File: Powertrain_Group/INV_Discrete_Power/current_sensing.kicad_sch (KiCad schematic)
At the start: 5 parts, among them U1 CKSR_75-NP

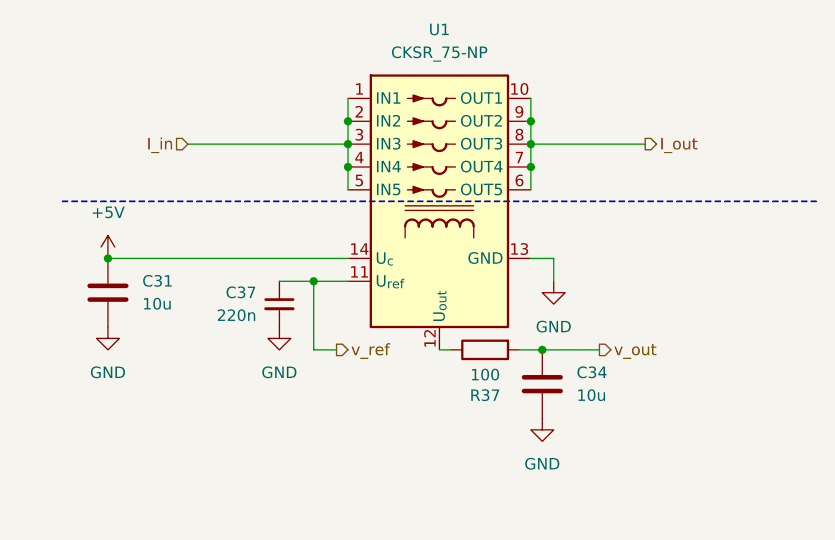
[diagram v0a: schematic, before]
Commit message: [INV_Discrete_Power] V1.1 by Jack Kuo
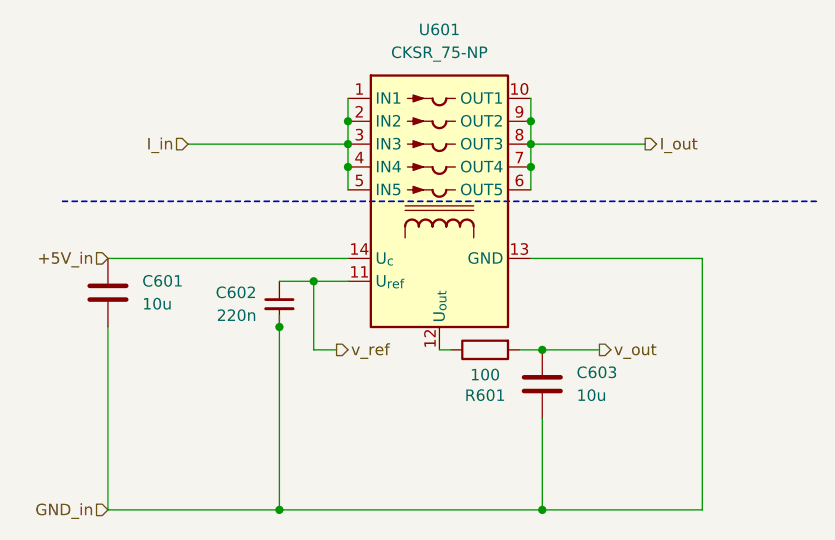
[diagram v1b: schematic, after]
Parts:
- renumbered C31 to C601, C37 to C602, C34 to C603, R37 to R601, U1 to U601
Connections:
- net +5V renamed +5V_in
- net GND renamed GND_in
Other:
- company: (none) -> NTURacing
- title: (none) -> INV_Discrete_Power

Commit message: [INV_Discrete_Power] V1.2
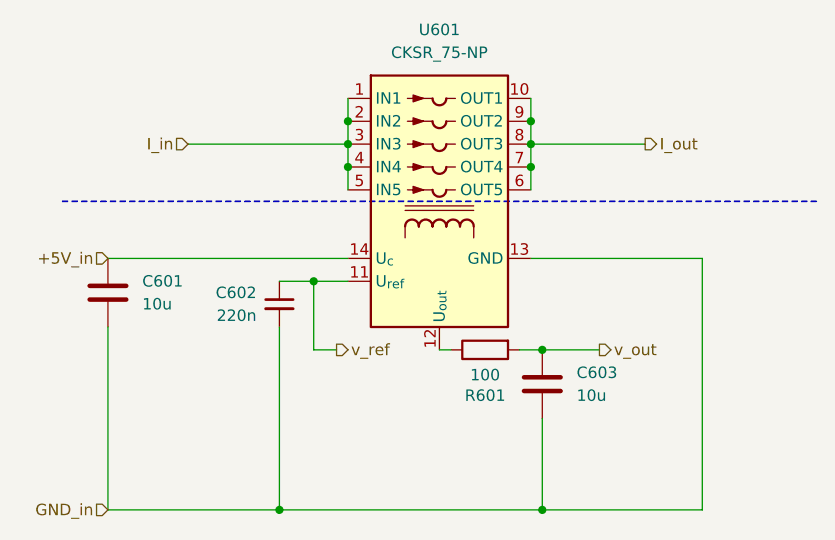
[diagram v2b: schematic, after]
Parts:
- U601: footprint Sensor_Current:LEM_CKSR -> nturt_kicad_lib_EP7:LEM_CKSR
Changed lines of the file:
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@@
 		(title "INV_Discrete_Power")
 		(date "2026-03-13")
-		(rev "1.1")
+		(rev "1.2")
 		(company "NTURacing")
 		(comment 1 "LY Chen")
@@
 		(color 0 0 0 0)
 	)
-	(junction
-		(at 116.84 86.36)
-		(diameter 0)
-		(color 0 0 0 0)
-	)
 	(wire
 		(pts
 			(xy 146.05 88.9) (xy 152.4 88.9)
-		)
-		(stroke
-			(width 0)
-			(type default)
-		)
-	)
-	(wire
-		(pts
-			(xy 116.84 85.09) (xy 116.84 86.36)
 		)
 		(stroke
@@
 			)
 		)
-		(property "Footprint" "Sensor_Current:LEM_CKSR"
+		(property "Footprint" "nturt_kicad_lib_EP7:LEM_CKSR"
 			(at 143.51 73.66 0)
 			(effects
